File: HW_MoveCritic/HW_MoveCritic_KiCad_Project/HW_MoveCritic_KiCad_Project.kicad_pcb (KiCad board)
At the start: 4 copper layers, 32.9 x 29 mm, 48 parts, among them J2 Conn_ARM_SWD_TagConnect_TC2030, J3 USB_C_Receptacle_USB2.0, SW1 SW_Push, U1 STM32WB55CEUx, U2 USBLC6-2P6, U3 MIC5365-3.3YD5, U5 BNO086, X1 32KHz768, X2 32MHz

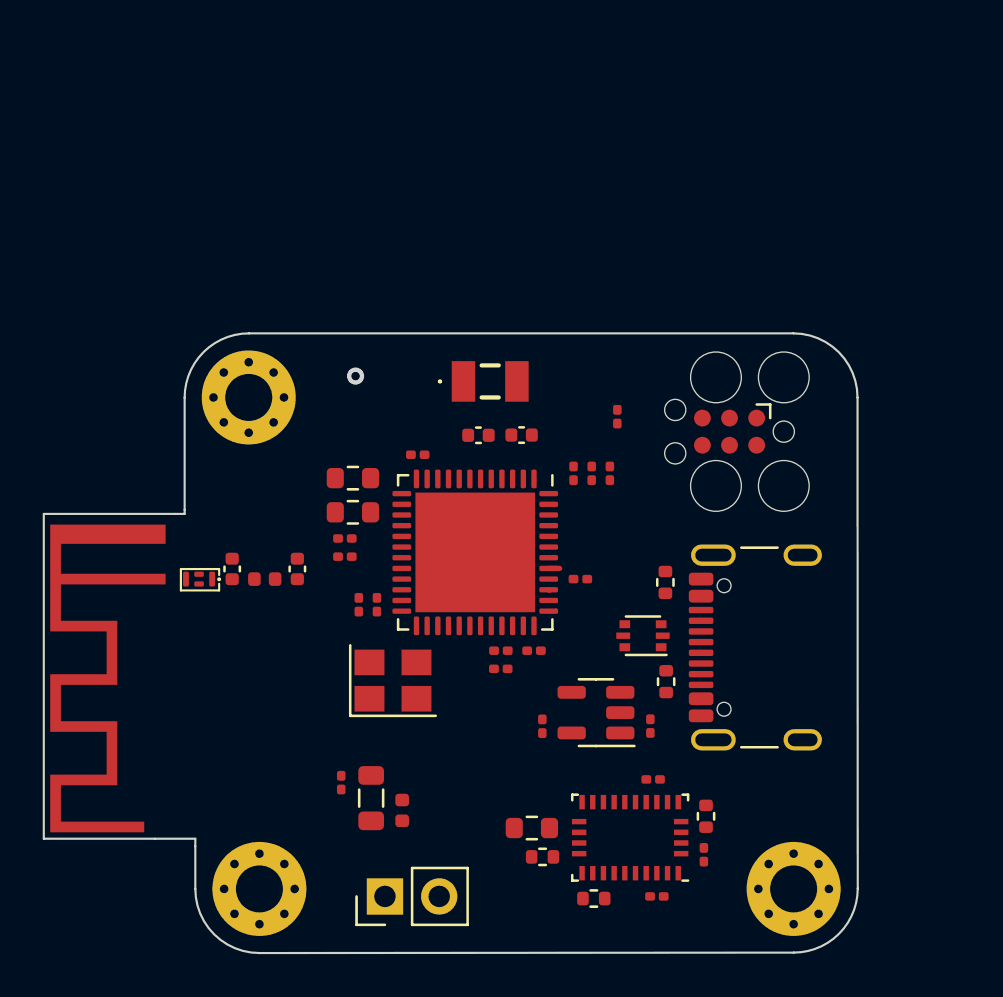
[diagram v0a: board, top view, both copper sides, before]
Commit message: Large Commit for HW design
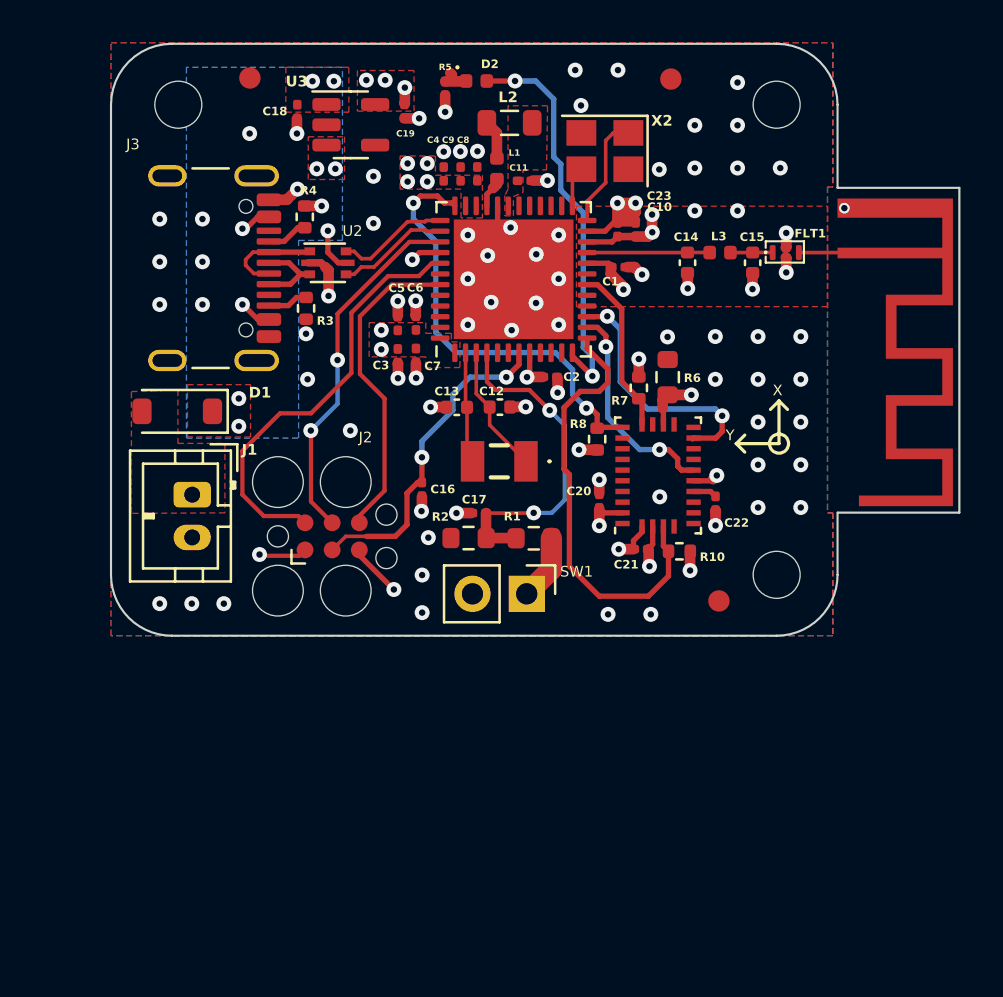
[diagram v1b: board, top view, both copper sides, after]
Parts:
- removed H3: MountingHole, MountingHole:MountingHole_2.2mm_M2_Pad_Via
- added D1: B5819W, Diode_SMD:D_SOD-123, F.Cu at (136.2, 91.7)
- added D2: LED, LED_SMD:LED_0402_1005Metric, F.Cu at (150.2, 76.2)
- added FID1: Fiducial, Fiducial:Fiducial_1mm_Mask2mm, F.Cu at (159.3, 76.1)
- added FID2: Fiducial, Fiducial:Fiducial_1mm_Mask2mm, F.Cu at (161.5, 100.5)
- added FID3: Fiducial, Fiducial:Fiducial_1mm_Mask2mm, F.Cu at (139.6, 76.0)
- added H4: MountingHole, MountingHole:MountingHole_2.2mm_M2_DIN965, F.Cu at (164.2, 99.3)
- added J1: JST_PH_2.00mm, Connector_JST:JST_PH_B2B-PH-K_1x02_P2.00mm_Vertical, F.Cu at (136.9, 95.5)
- added R5: 220R, Resistor_SMD:R_0201_0603Metric, F.Cu at (148.7, 76.5)
- AE1: footprint 830009678:2400MHz_PCB_Meander_Antenna -> 830009678:2400MHz_PCB_Inverted_F
- C1, C10, C2, C3, C4, C5, C6, C8: value 100n -> 0u1
- H1, H2: footprint MountingHole:MountingHole_2.2mm_M2_Pad_Via -> MountingHole:MountingHole_2.2mm_M2_DIN965
- U1: value STM32WB55CEUx -> STM32WB55CEU6
- moved AE1 38.5 mm to (172.8, 88.7)
- moved H2 36.9 mm to (136.2, 77.3), turned to -90 degrees
- moved C18 33.2 mm to (141.8, 77.6), turned to -90 degrees
- moved J3 32.8 mm to (136.8, 84.9), turned to -90 degrees
- moved L2 32.3 mm to (151.7, 78.2), turned to 0 degrees
- moved FLT1 31.4 mm to (164.6, 84.2), turned to 0 degrees
- moved L1 30.4 mm to (151.1, 80.3), turned to 90 degrees
- moved U3 29.8 mm to (144.3, 78.2), turned to 0 degrees
- moved C19 29.5 mm to (146.8, 77.6), turned to -90 degrees
- moved C11 29.4 mm to (152.4, 80.9), turned to 0 degrees
- moved C15 28.3 mm to (163.1, 84.7), turned to -90 degrees
- moved H1 28.2 mm to (164.2, 77.3), turned to -90 degrees
- moved R4 27.6 mm to (142.1, 82.6), turned to 90 degrees
- moved X2 26.7 mm to (156.2, 79.5), turned to 180 degrees
- moved L3 26.2 mm to (161.6, 84.2), turned to 0 degrees
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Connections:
- net Net-(U2-VBUS) renamed +5V
- U1 pad 12: unconnected-(U1-PA3-Pad12) -> Net-(D2-A)
- U1 pad 13: unconnected-(U1-PA4-Pad13) -> BNO_NBOOT
- U1 pad 14: unconnected-(U1-PA5-Pad14) -> BNO_NRST
- U1 pad 15: unconnected-(U1-PA6-Pad15) -> BNO_NINT
- U1 pad 45: BNO_NINT -> unconnected-(U1-PB5-Pad45)
- U1 pad 46: BNO_NRST -> unconnected-(U1-PB6-Pad46)
- U1 pad 47: BNO_NBOOT -> unconnected-(U1-PB7-Pad47)
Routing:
- net GND: track 0.00 -> 31.1 mm, vias 1 -> 89
- net +3.3V: track 0.00 -> 27.3 mm, vias 0 -> 22
- net BNO_NBOOT: track 0.00 -> 20.6 mm
- net I2C1_SDA: track 0.00 -> 20.4 mm, vias 0 -> 2
- net /SWDIO: track 0.51 -> 20.1 mm
- net Net-(D2-A): track 0.00 -> 18.7 mm, vias 0 -> 2
- net /SWCLK: track 0.35 -> 16.9 mm, vias 0 -> 2
- net /BOOT_0: track 0.00 -> 16.0 mm, vias 0 -> 2
- net NRST: track 0.04 -> 15.3 mm, vias 0 -> 2
- net /SWO: track 0.00 -> 15.0 mm
- net BNO_NINT: track 0.00 -> 12.0 mm, vias 0 -> 2
- net BNO_NRST: track 0.00 -> 10.1 mm, vias 0 -> 2
- net I2C1_SCL: track 0.00 -> 7.89 mm
- net /LSE_OUT: track 0.00 -> 6.05 mm
- net RF1: track 0.00 -> 5.74 mm
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- added copper zone on B.Cu, net +3.3V
- added copper zone on F.Cu, net +3.3V
- added copper zone on B.Cu, net +5V
- added copper zone on F.Cu, net +5V
- added copper zone on F.Cu, net /SMPSFB
- added copper zone on F.Cu, net /VIN
- added copper zone on F.Cu, net GND
- added copper zone on In2.Cu, net GND
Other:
- board size 32.9 x 29 mm -> 34 x 27.7 mm
- rule pad_to_mask_clearance: 0.08 -> 0
- board text added: "MoveCritic FBTM REV A AC 03/24"
- board text added: "X"
- board text added: "Y"
